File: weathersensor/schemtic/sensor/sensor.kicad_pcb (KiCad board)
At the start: 2 copper layers, 1 part, among them U1 ESP32-DEVKITC-32D

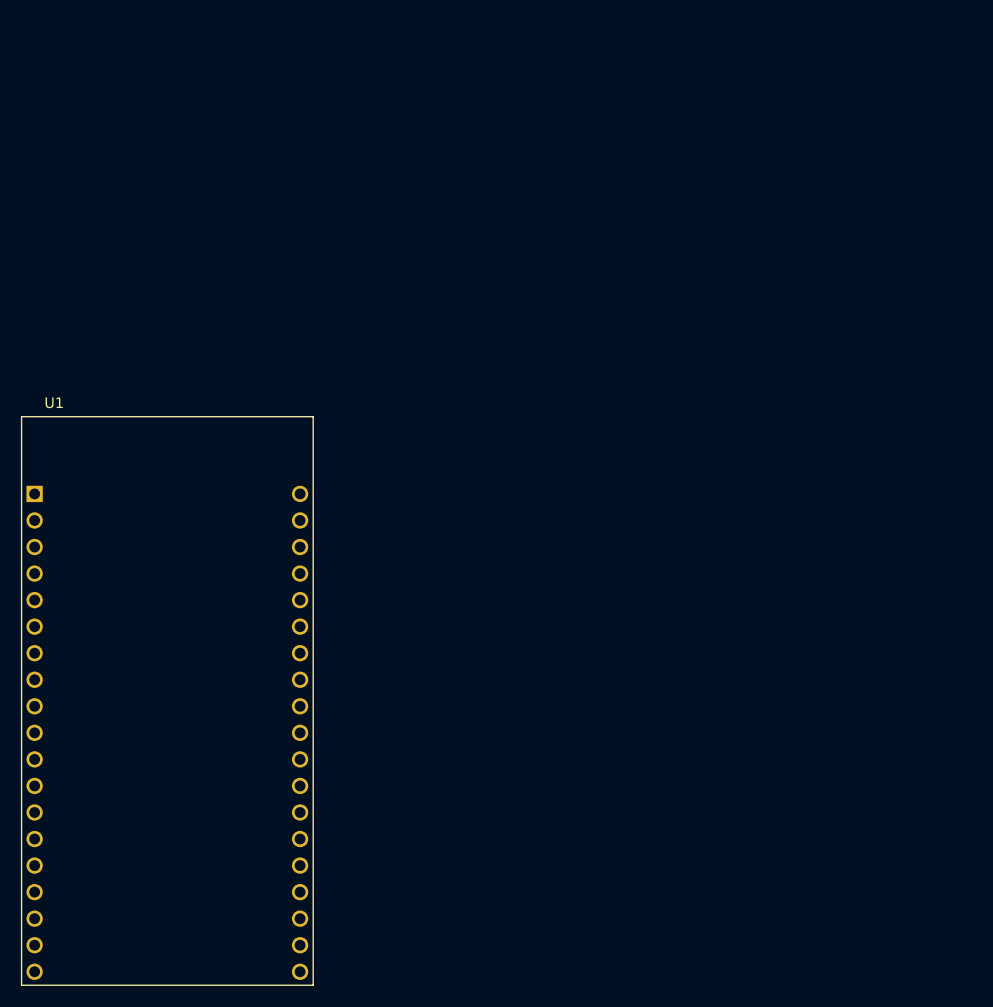
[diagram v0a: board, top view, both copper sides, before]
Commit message: Start commit message
21.03.2023
	- create and pcb for weathersensor

22.02.2023
	- add schematic and pcb for mqtt_wlan_bridge
	- remove old from git repo

	TODO:
	- create schematic and pcb for weathersensor
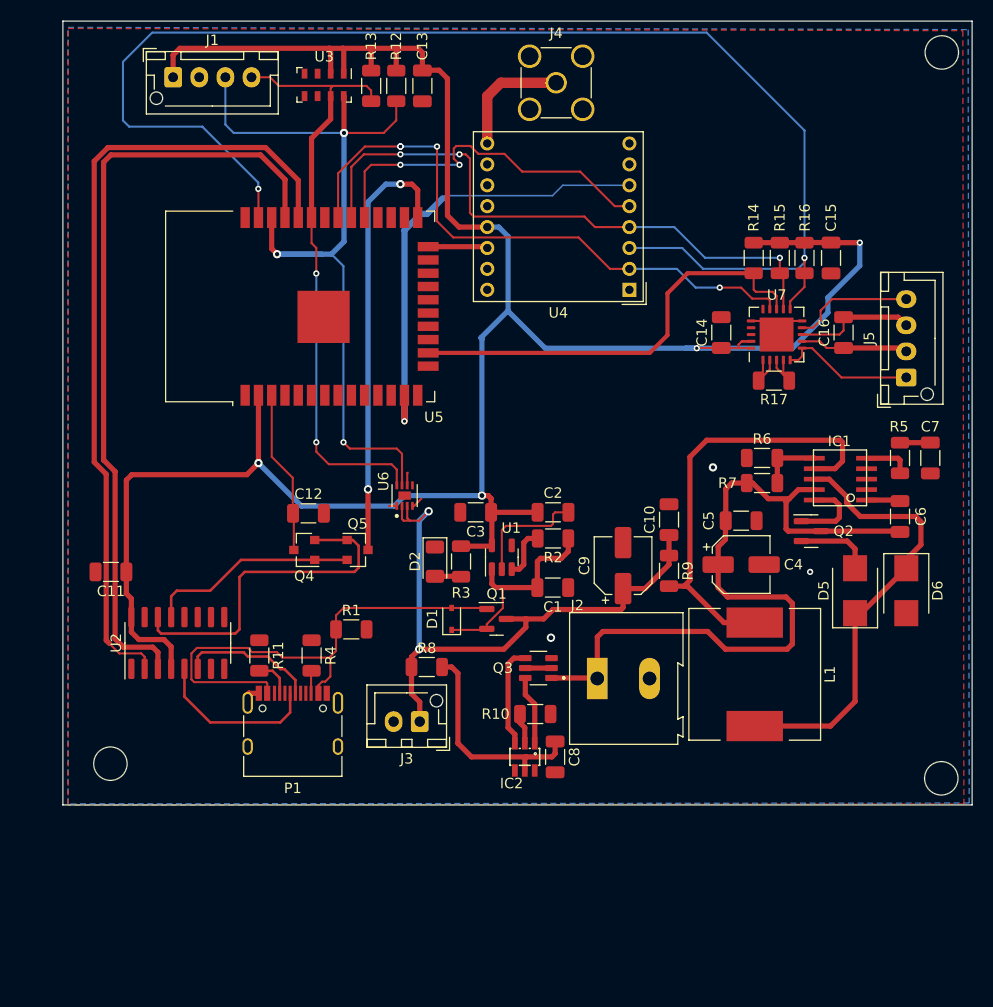
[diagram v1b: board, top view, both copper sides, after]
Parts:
- added ?: , , F.Cu at (175.1, 18.0)
- added ?: , , F.Cu at (175.1, 87.5)
- added C1: 1.0u, Capacitor_SMD:C_1206_3216Metric, F.Cu at (137.9, 69.2)
- added C10: 220n, Capacitor_SMD:C_1206_3216Metric, F.Cu at (149.0, 62.7)
- added C11: 100n, Capacitor_SMD:C_1206_3216Metric, F.Cu at (95.6, 67.7)
- added C12: 1u, Capacitor_SMD:C_1206_3216Metric, F.Cu at (114.5, 62.1)
- added C13: 100n, Capacitor_SMD:C_1206_3216Metric, F.Cu at (125.4, 21.2)
- added C14: 0.1u, Capacitor_SMD:C_1206_3216Metric, F.Cu at (154.0, 44.8)
- added C15: 0.1u, Capacitor_SMD:C_1206_3216Metric, F.Cu at (164.5, 37.7)
- added C16: 10n, Capacitor_SMD:C_1206_3216Metric, F.Cu at (165.7, 44.8)
- added C2: 1.0u, Capacitor_SMD:C_1206_3216Metric, F.Cu at (137.9, 62.0)
- added C3: 10u, Capacitor_SMD:C_1206_3216Metric, F.Cu at (130.5, 62.0)
- added C4: 47u/16V, Capacitor_SMD:CP_Elec_5x5.3, F.Cu at (155.9, 67.0)
- added C5: 10n, Capacitor_SMD:C_1206_3216Metric, F.Cu at (155.9, 62.8)
- added C6: 100n, Capacitor_SMD:C_1206_3216Metric, F.Cu at (171.1, 62.4)
- added C7: 22n, Capacitor_SMD:C_1206_3216Metric, F.Cu at (174.0, 56.8)
- added C8: 100n, Capacitor_SMD:C_1206_3216Metric, F.Cu at (138.1, 85.4)
- added C9: 47u/16V, Capacitor_SMD:CP_Elec_5x5.3, F.Cu at (144.6, 67.1)
- added D1: BAT60A, Diode_SMD:D_SOD-323, F.Cu at (128.2, 72.2)
- added D2: LED, LED_SMD:LED_1206_3216Metric, F.Cu at (126.6, 66.7)
- added D5: SSB43L, Diode_SMD:D_SMB, F.Cu at (166.8, 69.5)
- added D6: SSB43L, Diode_SMD:D_SMB, F.Cu at (171.7, 69.5)
- added IC1: CN3791, CN3791:SSOP10, F.Cu at (167.9, 58.8)
- added IC2: DW01A, DW01A:SOT23-6, F.Cu at (135.2, 85.4)
- added J1: I2C, Connector_JST:JST_XH_B4B-XH-AM_1x04_P2.50mm_Vertical, F.Cu at (101.5, 20.4)
- added J2: PANEL, TerminalBlock:TerminalBlock_Altech_AK300-2_P5.00mm, F.Cu at (142.1, 77.9)
- added J3: BAT, Connector_JST:JST_XH_B2B-XH-AM_1x02_P2.50mm_Vertical, F.Cu at (125.2, 82.0)
- added J4: ANT, Connector_Coaxial:SMA_Amphenol_901-144_Vertical, F.Cu at (138.2, 20.9)
- added J5: PT1000, Connector_JST:JST_XH_B4B-XH-AM_1x04_P2.50mm_Vertical, F.Cu at (171.7, 49.1)
- added L1: 82u, Inductor_SMD:L_12x12mm_H8mm, F.Cu at (157.2, 77.5)
- added P1: USB_C_Plug_USB2.0, Connector_USB:USB_C_Receptacle_HRO_TYPE-C-31-M-12, F.Cu at (113.0, 83.4)
- added Q1: IRLML6401, Package_TO_SOT_SMD:SOT-23, F.Cu at (132.5, 72.2)
- added Q2: AO3401A, Package_TO_SOT_SMD:SOT-23, F.Cu at (162.6, 63.8)
- added Q3: FS8205, FS8205:SOT95P280X145-6N, F.Cu at (136.5, 76.9)
- added Q4: BSS138, Package_TO_SOT_SMD:SOT-23, F.Cu at (114.1, 65.6)
- added Q5: BSS138, Package_TO_SOT_SMD:SOT-23, F.Cu at (119.2, 65.6)
- added R1: 10k, Resistor_SMD:R_1206_3216Metric, F.Cu at (118.6, 73.2)
- added R10: 1k, Resistor_SMD:R_1206_3216Metric, F.Cu at (136.2, 81.3)
- added R11: 5k1, Resistor_SMD:R_1206_3216Metric, F.Cu at (109.8, 75.7)
- added R12: 10k, Resistor_SMD:R_1206_3216Metric, F.Cu at (122.9, 21.2)
- added R13: 10k, Resistor_SMD:R_1206_3216Metric, F.Cu at (120.5, 21.2)
- added R14: 10k, Resistor_SMD:R_1206_3216Metric, F.Cu at (157.1, 37.7)
- added R15: 10k, Resistor_SMD:R_1206_3216Metric, F.Cu at (159.6, 37.7)
- added R16: 10k, Resistor_SMD:R_1206_3216Metric, F.Cu at (162.0, 37.7)
- added R17: 4k 1% or better, Resistor_SMD:R_1206_3216Metric, F.Cu at (159.0, 49.4)
- added R2: 10k, Resistor_SMD:R_1206_3216Metric, F.Cu at (137.9, 64.5)
- added R3: 1k, Resistor_SMD:R_1206_3216Metric, F.Cu at (129.1, 66.7)
- added R4: 5k1, Resistor_SMD:R_1206_3216Metric, F.Cu at (114.8, 75.7)
- added R5: 120, Resistor_SMD:R_1206_3216Metric, F.Cu at (171.1, 56.8)
- added R6: 22k, Resistor_SMD:R_1206_3216Metric, F.Cu at (157.9, 56.8)
- added R7: 178k, Resistor_SMD:R_1206_3216Metric, F.Cu at (157.9, 59.2)
- added R8: 100, Resistor_SMD:R_1206_3216Metric, F.Cu at (125.8, 76.8)
- added R9: 0.05, Resistor_SMD:R_1206_3216Metric, F.Cu at (149.0, 67.6)
- added REF**: MountingHole_3.2mm_M3, MountingHole:MountingHole_3.2mm_M3, F.Cu at (95.5, 86.0)
- added U2: CH340C, Package_SO:SOIC-16_3.9x9.9mm_P1.27mm, F.Cu at (102.0, 74.5)
- added U3: MS5611-01BA, Package_LGA:LGA-8_3x5mm_P1.25mm, F.Cu at (116.0, 21.1)
- added U4: RFM95W-868S2, RF_Module:HOPERF_RFM9XW_THT, F.Cu at (145.2, 40.7)
- added U5: ESP32-WROOM-32D, RF_Module:ESP32-WROOM-32, F.Cu at (116.7, 42.3)
- added U6: MAX17048G, MAX17048G:SON50P200X200X80-9N, F.Cu at (123.7, 60.4)
- added U7: MAX31865xTP, Package_DFN_QFN:TQFN-20-1EP_5x5mm_P0.65mm_EP3.25x3.25mm, F.Cu at (159.3, 45.0)
- U1: value ESP32-DEVKITC-32D -> XC6220B331MR; footprint ESP32-DEVKITC-32D:MODULE_ESP32-DEVKITC-32D -> Package_TO_SOT_SMD:SOT-23-5
- moved U1 34.8 mm to (133.0, 66.3), turned to 90 degrees
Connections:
- U1 pad 1: unconnected-(U1-Pad1) -> Net-(C1-Pad2)
- U1 pad 2: unconnected-(U1-Pad2) -> GND
- U1 pad 3: unconnected-(U1-Pad3) -> Net-(R2-Pad2)
- U1 pad 5: unconnected-(U1-Pad5) -> +3.3V
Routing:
- net +3.3V: track 0.00 -> 223.9 mm, vias 0 -> 4
- net MOSI: track 0.00 -> 130.6 mm, vias 0 -> 2
- net SCL: track 0.00 -> 79.9 mm, vias 0 -> 3
- net ESP32_RX: track 0.00 -> 76.9 mm
- net ESP32_TX: track 0.00 -> 74.5 mm
- net VSS: track 0.00 -> 73.3 mm
- net V_BAT: track 0.00 -> 60.6 mm, vias 0 -> 2
- net SDA: track 0.00 -> 58.9 mm, vias 0 -> 2
- net SCK: track 0.00 -> 58.5 mm, vias 0 -> 3
- net MISO: track 0.00 -> 57.7 mm, vias 0 -> 5
- net V_USB: track 0.00 -> 47.8 mm
- net RFM_RESET: track 0.00 -> 44.1 mm, vias 0 -> 1
- net Net-(D5-Pad1): track 0.00 -> 43.0 mm
- net Net-(IC1-Pad7): track 0.00 -> 42.4 mm
- net MAX_CS: track 0.00 -> 41.9 mm
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- added copper zone on B.Cu, net GND
- added copper zone on F.Cu, net GND
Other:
- board outline added: 87 x 75 mm
